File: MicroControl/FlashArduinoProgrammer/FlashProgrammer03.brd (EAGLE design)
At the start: 49.5 x 23.5 mm, 11 parts, among them U1 VREG-LD2985, X1 POGOPIN, X2 POGOPIN, X3 POGOPIN, X4 POGOPIN, X5 POGOPIN, X6 POGOPIN, X7 POGOPIN, X8 POGOPIN

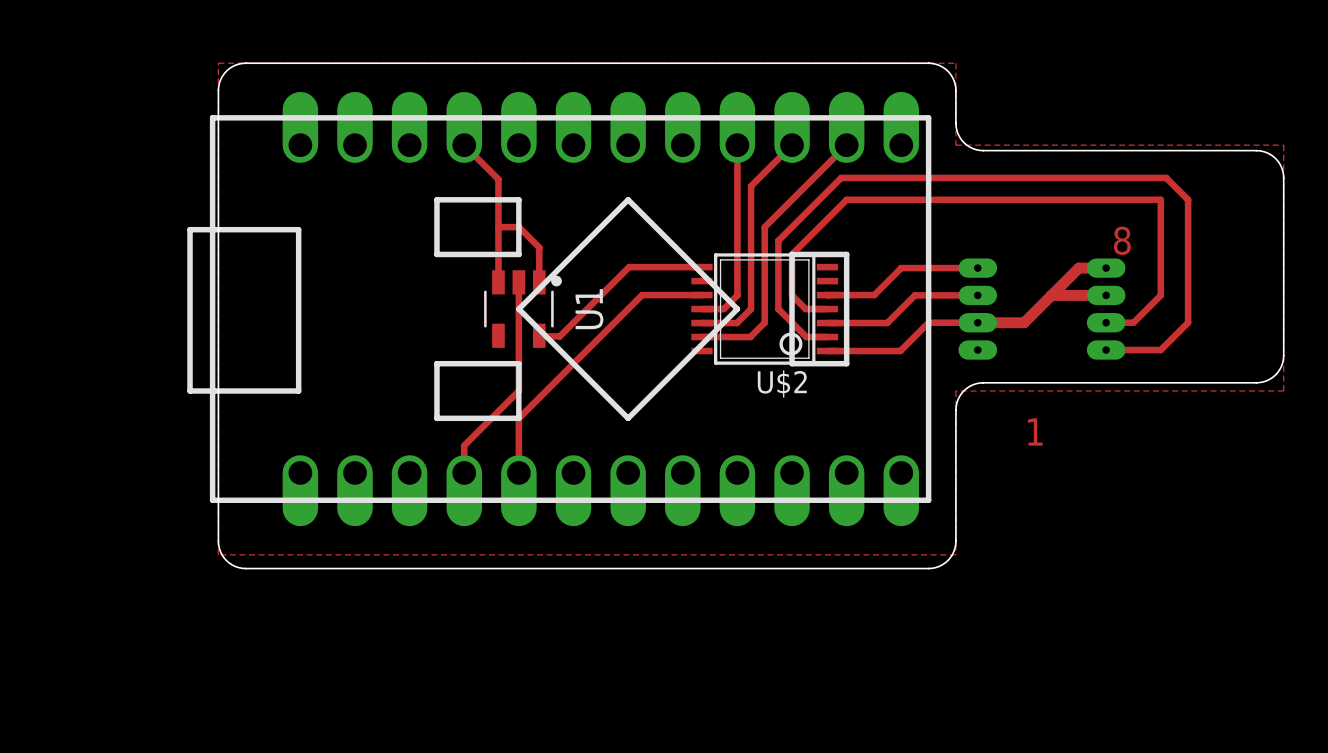
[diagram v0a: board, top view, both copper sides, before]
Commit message: _
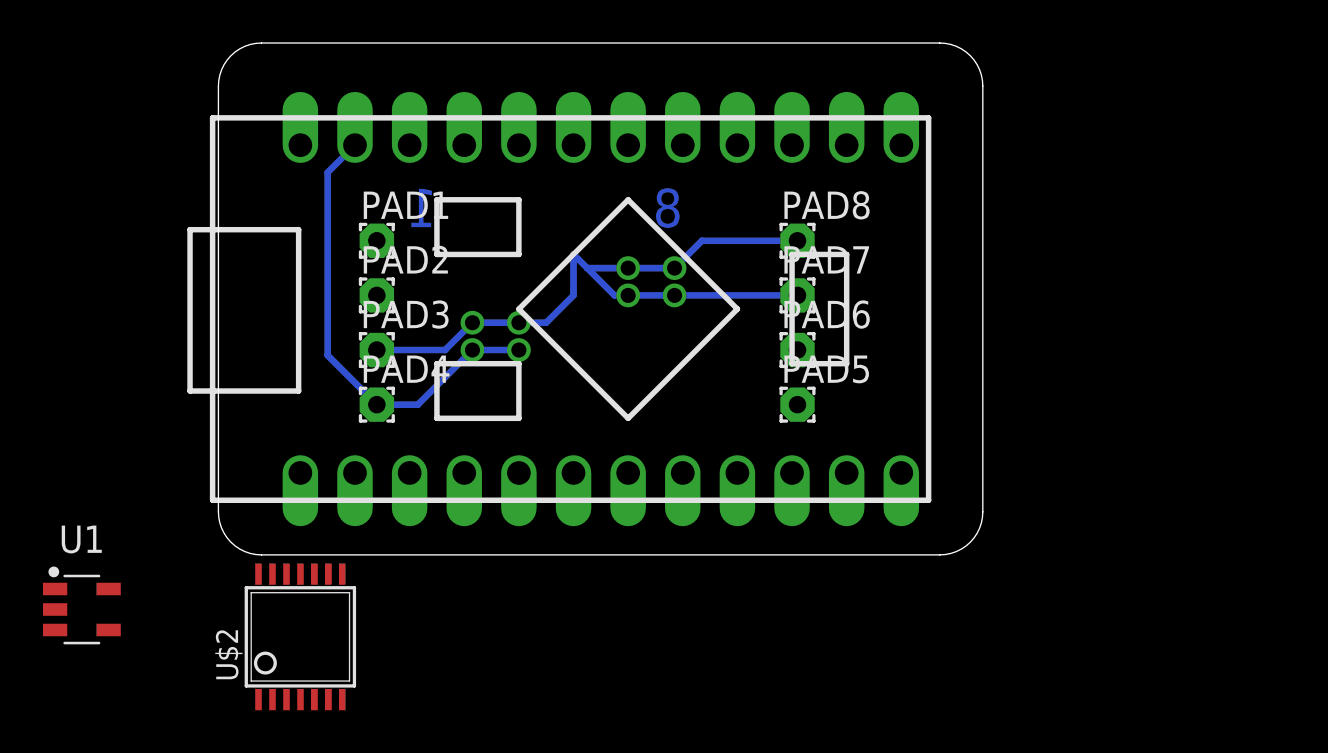
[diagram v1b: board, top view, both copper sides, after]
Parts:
- removed X1, X2, X3, X4, X5, X6, X7, X8: POGOPIN, Flamberm:POGOPIN
- added PAD1, PAD2, PAD3, PAD4, PAD5, PAD6, PAD7, PAD8: (no value), wirepad:1,6/0,8
- moved U$2 26.4 mm to (3.81, -3.81), turned to 0 degrees
- moved U1 24.7 mm to (-6.35, -2.54), turned to 0 degrees
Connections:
- removed net N$7 (its old number): U$2.2, X5.P$1
- removed net P2: U$2.3, X2.P$1
- removed net P3,P8,P7: U$2.1, U$2.8, U1.5, X3.P$1, X7.P$1, X8.P$1
- new net N$10: PAD5.1, U$2.4
- new net N$11: PAD1.1, U$2.5
- new net N$6: U$1.16, U$2.11
- new net N$9: PAD2.1, U$2.3
- net GND: no longer U$1.GND@1, U$2.7, U1.2, X4.P$1
- net N$2: now also PAD4.1, U$1.GND@1, U$2.7, U1.2; no longer U$1.15, U$2.11
- net N$3: now also U$1.15; no longer U$1.16
- net N$4: now also PAD3.1, PAD7.1, PAD8.1, U$2.1, U$2.8, U1.5; no longer U$2.5, X1.P$1
- net N$8: now also PAD6.1, U$2.2; no longer U$2.4, X6.P$1
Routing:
- net N$7 (its old number): track 36.7 -> 0.00 mm
- net N$8: track 29.5 -> 0.00 mm
- net N$4: track 7.53 -> 33.6 mm, vias 0 -> 6
- net P3,P8,P7: track 26.0 -> 0.00 mm
- net N$1: track 13.4 -> 0.00 mm
- net N$3: track 13.0 -> 0.00 mm
- net N$2: track 8.90 -> 21.2 mm, vias 0 -> 2
- net N$5: track 11.0 -> 0.00 mm
- net N$7: track 10.9 -> 0.00 mm
- net GND: track 9.91 -> 0.00 mm
- net P2: track 7.52 -> 0.00 mm
- removed copper zone on layer 1, net GND
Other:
- board size 49.5 x 23.5 mm -> 35.5 x 23.8 mm
